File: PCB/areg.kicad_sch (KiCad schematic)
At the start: 14 parts, among them J3 AREG, Q10 2N3906, Q9 2N5457, U2 LM324

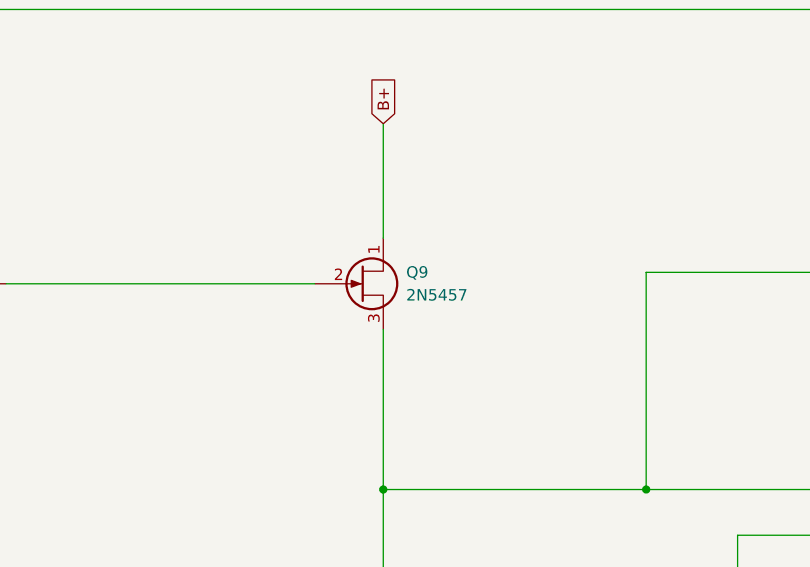
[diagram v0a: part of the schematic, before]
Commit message: Necessary Changes to Schematic and PCB
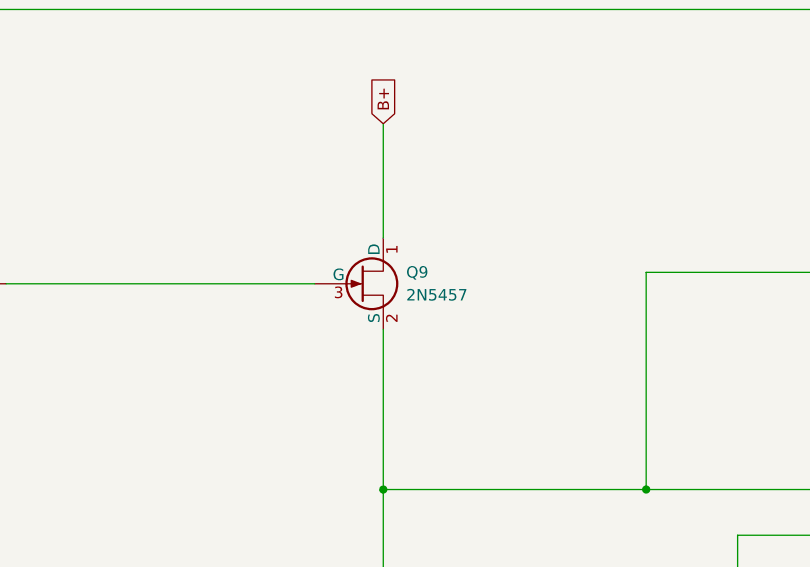
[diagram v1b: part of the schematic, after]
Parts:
- C18: footprint Capacitor_THT:CP_Radial_D4.0mm_P1.50mm -> Capacitor_THT:CP_Radial_D4.0mm_P2.00mm
- J3: footprint Connector_PinHeader_2.00mm:PinHeader_1x05_P2.00mm_Vertical -> Connector_PinSocket_2.54mm:PinSocket_1x05_P2.54mm_Vertical
- Q10: footprint Package_TO_SOT_THT:TO-92_Inline -> Package_TO_SOT_THT:TO-92_Inline_Wide
- Q9: footprint Package_TO_SOT_THT:TO-92_Inline -> Package_TO_SOT_THT:TO-92_Inline_Wide; symbol Device:Q_NJFET_DGS -> Device:Q_NJFET_DSG
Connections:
- net X18: now also Q9.2 (S); no longer Q9.3 (S)
- net at R52.2: now also Q9.3 (G); no longer Q9.2 (G)
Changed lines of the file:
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@@
 			)
 		)
-		(property "Footprint" "Capacitor_THT:CP_Radial_D4.0mm_P1.50mm"
+		(property "Footprint" "Capacitor_THT:CP_Radial_D4.0mm_P2.00mm"
 			(at 39.0652 127 0)
 			(hide yes)
@@
 	)
 	(symbol
-		(lib_id "Device:Q_NJFET_DGS")
+		(lib_id "Device:Q_NJFET_DSG")
 		(at 123.19 107.95 0)
 		(unit 1)
@@
 		(fields_autoplaced yes)
 		(property "Reference" "Q9"
-			(at 128.27 106.68 0)
+			(at 128.27 106.6799 0)
 			(show_name no)
 			(do_not_autoplace no)
@@
 		)
 		(property "Value" "2N5457"
-			(at 128.27 109.22 0)
+			(at 128.27 109.2199 0)
 			(show_name no)
 			(do_not_autoplace no)
@@
 			)
 		)
-		(property "Footprint" "Package_TO_SOT_THT:TO-92_Inline"
+		(property "Footprint" "Package_TO_SOT_THT:TO-92_Inline_Wide"
 			(at 128.27 105.41 0)
 			(hide yes)
@@
 			)
 		)
-		(property "Description" ""
+		(property "Description" "N-JFET transistor, drain/source/gate"
 			(at 123.19 107.95 0)
 			(hide yes)
@@
 			)
 		)
-		(property "Footprint" "Package_TO_SOT_THT:TO-92_Inline"
+		(property "Footprint" "Package_TO_SOT_THT:TO-92_Inline_Wide"
 			(at 167.64 52.705 0)
 			(hide yes)
@@
 			)
 		)
-		(property "Footprint" "Connector_PinHeader_2.00mm:PinHeader_1x05_P2.00mm_Vertical"
+		(property "Footprint" "Connector_PinSocket_2.54mm:PinSocket_1x05_P2.54mm_Vertical"
 			(at 261.62 67.31 0)
 			(hide yes)
